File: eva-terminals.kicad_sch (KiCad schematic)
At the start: 24 parts, among them J1 RIBBON, J4 EXTRUDER, J5 HEATER, J6 SPI, J7 AUX, U1 LD39015M33R, U2 ADXL345

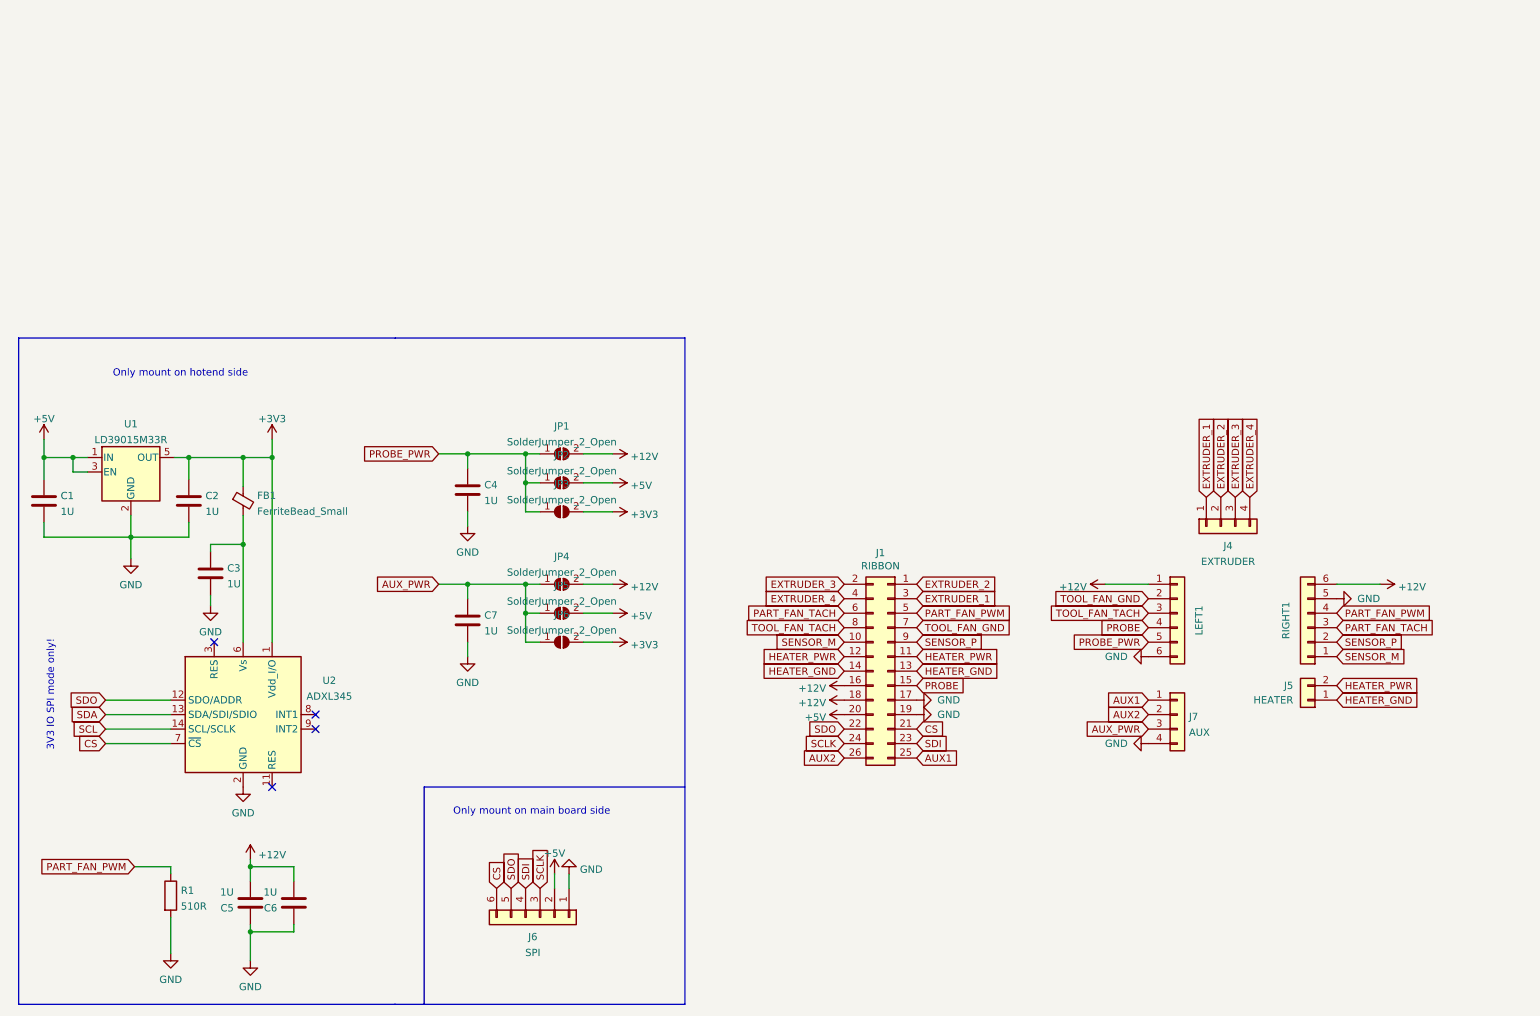
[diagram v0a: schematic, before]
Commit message: wip dual ribbon
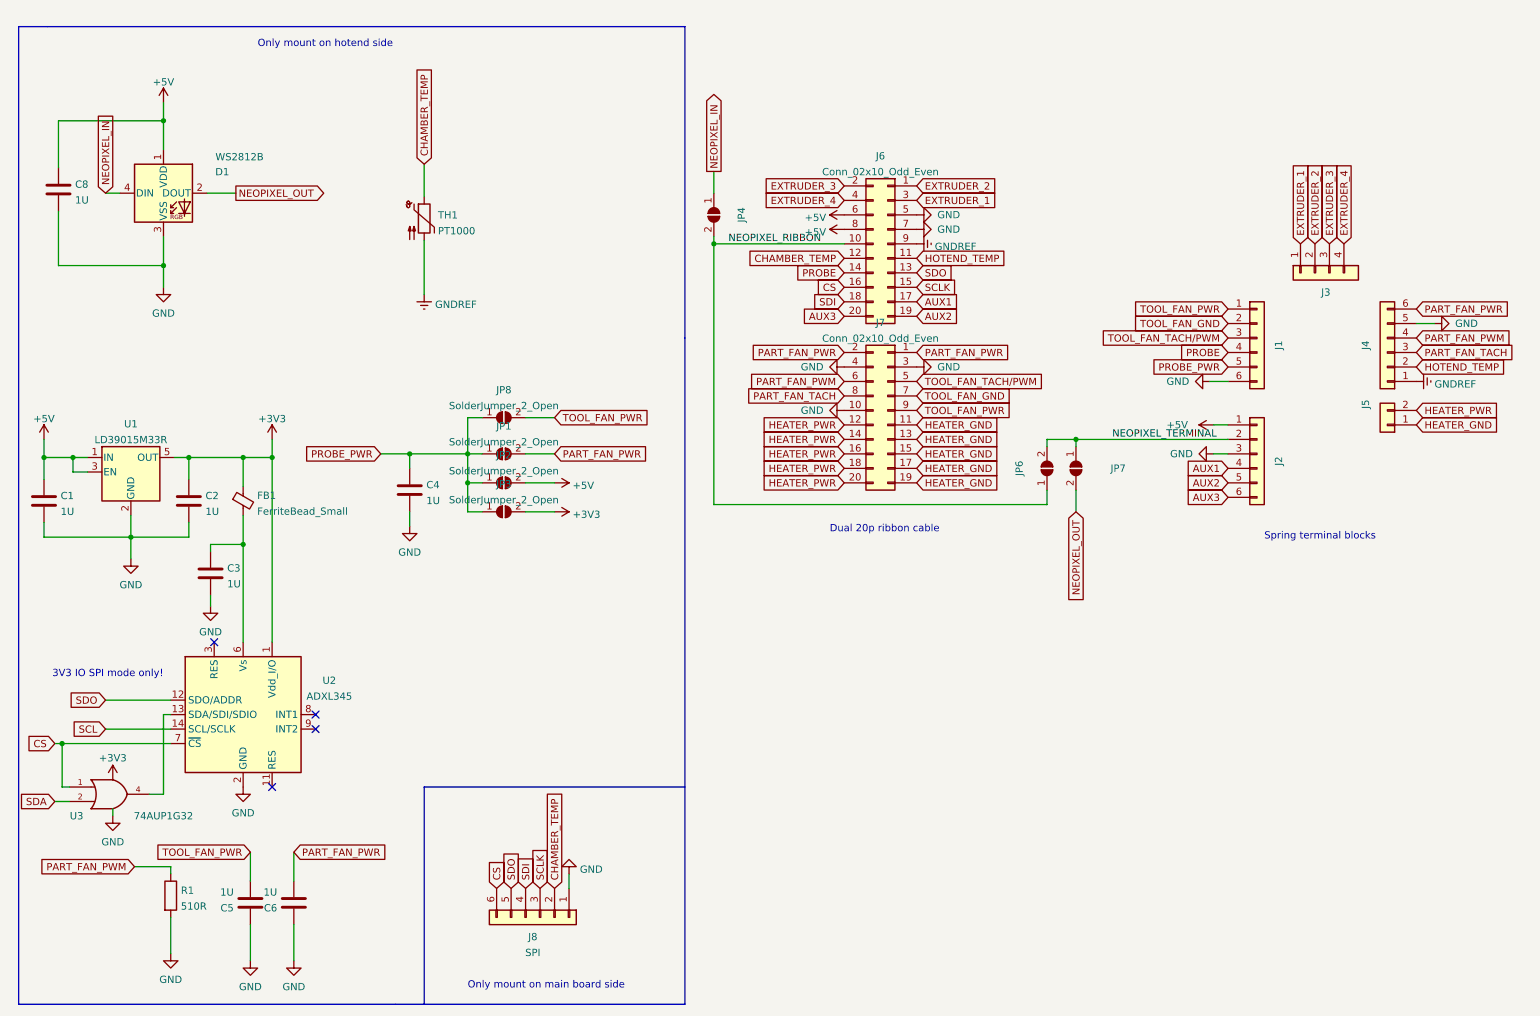
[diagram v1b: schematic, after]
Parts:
- removed C7: 1U, Capacitor_SMD:C_0805_2012Metric, symbol Device:C
- removed J1: RIBBON, Eagle_WR-MM (rev20b):690367292676, symbol Connector_Generic:Conn_02x13_Odd_Even
- removed J4: EXTRUDER, Eagle_WR-TBL Spring Clamp (rev21a):691402910004B, symbol eva-terminals:Conn_01x04_dual
- removed J7: AUX, Eagle_WR-TBL Spring Clamp (rev21a):691403900004B, symbol eva-terminals:Conn_01x04_dual
- removed JP5: SolderJumper_2_Open, Jumper:SolderJumper-2_P1.3mm_Open_RoundedPad1.0x1.5mm, symbol Jumper:SolderJumper_2_Open
- added C8: 1U, Capacitor_SMD:C_0805_2012Metric, symbol Device:C
- added D1: WS2812B, LED_SMD:LED_WS2812B_PLCC4_5.0x5.0mm_P3.2mm, symbol LED:WS2812B
- added J2: 691403900006B, Eagle_WR-TBL Spring Clamp (rev21a):691403900006B, symbol eva-terminals:Conn_01x06_dualpin
- added J3: Conn_01x04_dualpin, Eagle_WR-TBL Spring Clamp (rev21a):691402910004B, symbol eva-terminals:Conn_01x04_dualpin
- added J6, J7: Conn_02x10_Odd_Even, Eagle_WR-MM (rev20b):690367292076, symbol Connector_Generic:Conn_02x10_Odd_Even
- added JP7, JP8: SolderJumper_2_Open, Jumper:SolderJumper-2_P1.3mm_Open_RoundedPad1.0x1.5mm, symbol Jumper:SolderJumper_2_Open
- added TH1: PT1000, Resistor_SMD:R_1206_3216Metric, symbol Sensor_Temperature:PT1000
- added U3: 74AUP1G32, Package_TO_SOT_SMD:SOT-553, symbol 74xGxx:74AUP1G32
- renumbered LEFT1 to J1, RIGHT1 to J4, J6 to J8
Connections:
- net +3V3: now also U3.5 (VCC); no longer JP6.2 (B)
- net +5V: now also C8.1, D1.1 (VDD), J2.1 (Pin_1), J2.A1 (Pin_1A), J6.6 (Pin_6), J6.8 (Pin_8); no longer J8.2 (Pin_2), J8.A2 (Pin_A2)
- net AUX1: now also J2.4 (Pin_4), J2.A4 (Pin_A4), J6.17 (Pin_17)
- net AUX2: now also J2.5 (Pin_5), J2.A5 (Pin_A5), J6.19 (Pin_19)
- net CS: now also J6.16 (Pin_16), U3.1
- net EXTRUDER_1: now also J3.1 (Pin_1), J3.A1 (Pin_1A), J6.3 (Pin_3)
- net EXTRUDER_2: now also J3.2 (Pin_2), J3.A2 (Pin_A2), J6.1 (Pin_1)
- net EXTRUDER_3: now also J3.3 (Pin_3), J3.A3 (Pin_3), J6.2 (Pin_2)
- net EXTRUDER_4: now also J3.4 (Pin_4), J3.A4 (Pin_A4), J6.4 (Pin_4)
- net GND: now also C8.2, D1.3 (VSS), J2.3 (Pin_3), J2.A3 (Pin_3), J6.5 (Pin_5), J6.7 (Pin_7), J7.10 (Pin_10), J7.3 (Pin_3), J7.4 (Pin_4), U3.3 (GND)
- net HEATER_GND: now also J7.11 (Pin_11), J7.13 (Pin_13), J7.15 (Pin_15), J7.17 (Pin_17), J7.19 (Pin_19)
- net HEATER_PWR: now also J7.12 (Pin_12), J7.14 (Pin_14), J7.16 (Pin_16), J7.18 (Pin_18), J7.20 (Pin_20)
- net PART_FAN_PWM: now also J7.6 (Pin_6)
- net PART_FAN_TACH: now also J7.8 (Pin_8)
- net PROBE: now also J6.14 (Pin_14)
- net PROBE_PWR: now also JP8.1 (A)
- net SCLK: now also J6.15 (Pin_15)
- net SDA: now also U3.2; no longer U2.13 (SDA/SDI/SDIO)
- net SDI: now also J6.18 (Pin_18)
- net SDO: now also J6.13 (Pin_13)
- net TOOL_FAN_GND: now also J7.7 (Pin_7)
- net +12V renamed PART_FAN_PWR
- net PART_FAN_PWR: now also J7.1 (Pin_1), J7.2 (Pin_2); no longer C5.2, J1.1 (Pin_1), J1.A1 (Pin_1A), JP4.2 (B)
- net AUX_PWR renamed NEOPIXEL_IN
- net NEOPIXEL_IN: now also D1.4 (DIN); no longer JP6.1 (A)
- net SENSOR_M renamed GNDREF
- net GNDREF: now also J6.9 (Pin_9), TH1.2
- net SENSOR_P renamed HOTEND_TEMP
- net HOTEND_TEMP: now also J6.11 (Pin_11)
- net TOOL_FAN_TACH renamed TOOL_FAN_TACH/PWM
- net TOOL_FAN_TACH/PWM: now also J7.5 (Pin_5)
- new net: U2.13 (SDA/SDI/SDIO), U3.4
- new net AUX3: J2.6 (Pin_6), J2.A6 (Pin_A6), J6.20 (Pin_20)
- new net CHAMBER_TEMP: J6.12 (Pin_12), J8.2 (Pin_2), J8.A2 (Pin_A2), TH1.1
- new net NEOPIXEL_OUT: D1.2 (DOUT), JP7.2 (B)
- new net NEOPIXEL_RIBBON: J6.10 (Pin_10), JP4.2 (B), JP6.1 (A)
- new net NEOPIXEL_TERMINAL: J2.2 (Pin_2), J2.A2 (Pin_A2), JP6.2 (B), JP7.1 (A)
- new net TOOL_FAN_PWR: C5.2, J1.1 (Pin_1), J1.A1 (Pin_1A), J7.9 (Pin_9), JP8.2 (B)
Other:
- note added: "Dual 20p ribbon cable"
- note added: "Spring terminal blocks"
- moved on the sheet: C4, J1, J4, J5, JP1, JP2, JP3

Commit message: finalized board layout rev 1
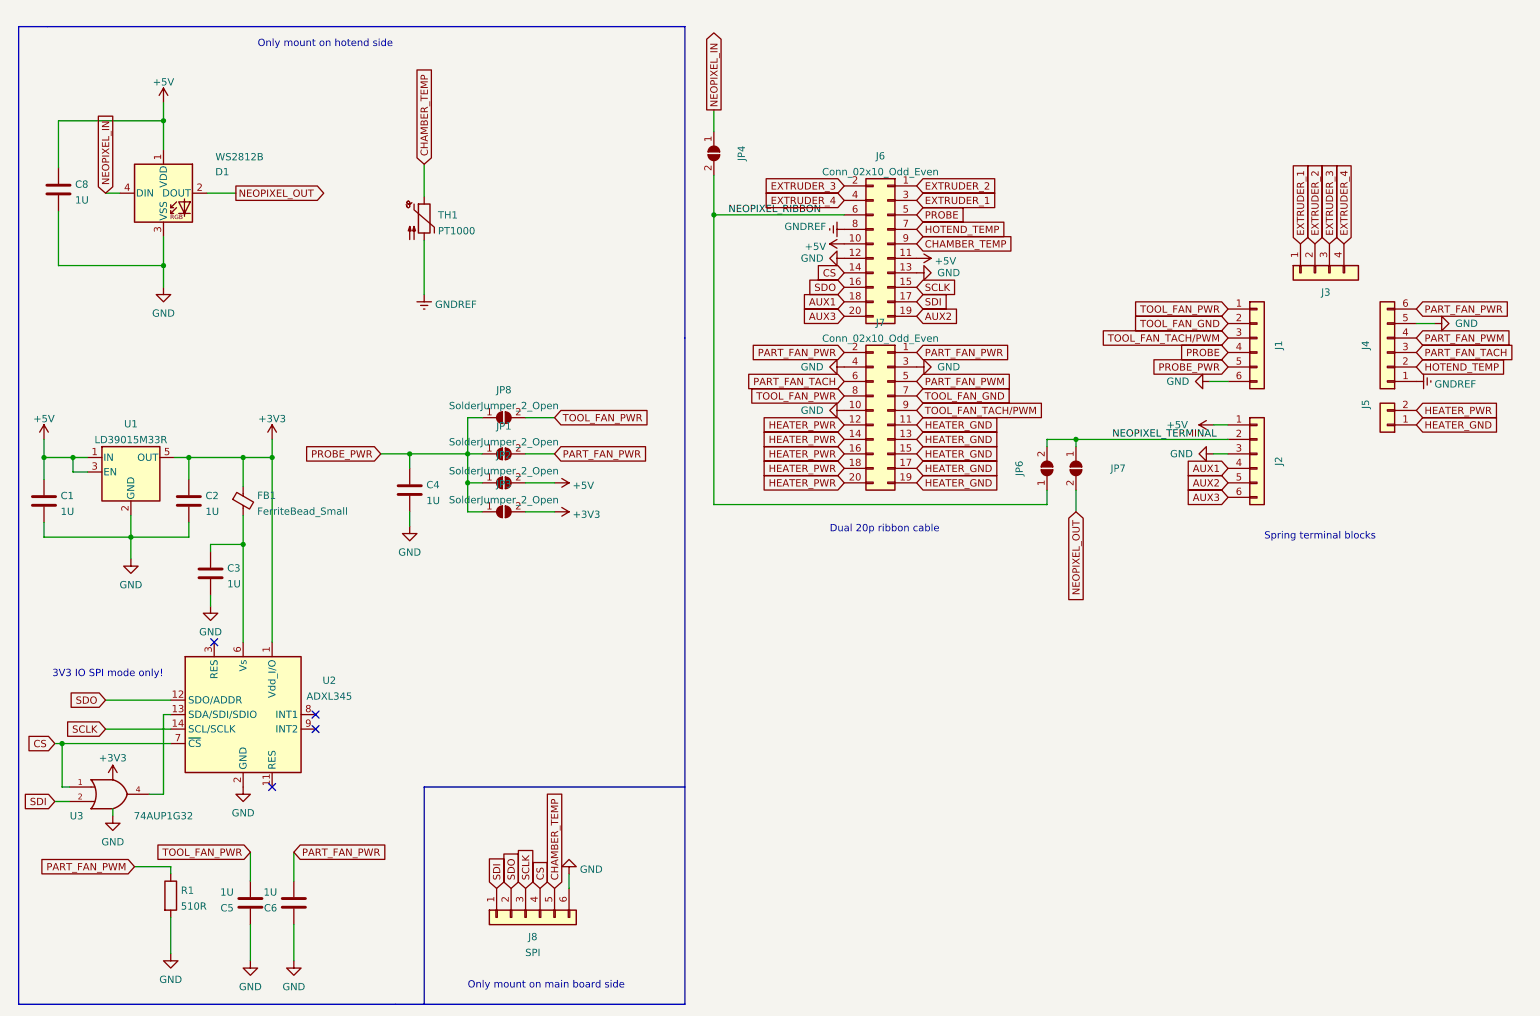
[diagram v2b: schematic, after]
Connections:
- net SCL is gone; now on net SCLK: U2.14 (SCL/SCLK)
- net SDA is gone; now on net SDI: U3.2
- net +5V: now also J6.10 (Pin_10), J6.11 (Pin_11); no longer J6.6 (Pin_6), J6.8 (Pin_8)
- net AUX1: now also J6.18 (Pin_18); no longer J6.17 (Pin_17)
- net CHAMBER_TEMP: now also J6.9 (Pin_9), J8.5 (Pin_5), J8.A5 (Pin_A5); no longer J6.12 (Pin_12), J8.2 (Pin_2), J8.A2 (Pin_A2)
- net CS: now also J6.14 (Pin_14), J8.4 (Pin_4), J8.A4 (Pin_A4); no longer J6.16 (Pin_16), J8.6 (Pin_6), J8.A6 (Pin_A6)
- net GND: now also J6.12 (Pin_12), J6.13 (Pin_13), J8.6 (Pin_6), J8.A6 (Pin_A6); no longer J6.5 (Pin_5), J6.7 (Pin_7), J8.1 (Pin_1), J8.A1 (Pin_1A)
- net GNDREF: now also J6.8 (Pin_8); no longer J6.9 (Pin_9)
- net HOTEND_TEMP: now also J6.7 (Pin_7); no longer J6.11 (Pin_11)
- net NEOPIXEL_RIBBON: now also J6.6 (Pin_6); no longer J6.10 (Pin_10)
- net PART_FAN_PWM: now also J7.5 (Pin_5); no longer J7.6 (Pin_6)
- net PART_FAN_TACH: now also J7.6 (Pin_6); no longer J7.8 (Pin_8)
- net PROBE: now also J6.5 (Pin_5); no longer J6.14 (Pin_14)
- net SDI: now also J6.17 (Pin_17), J8.1 (Pin_1), J8.A1 (Pin_1A); no longer J6.18 (Pin_18), J8.4 (Pin_4), J8.A4 (Pin_A4)
- net SDO: now also J6.16 (Pin_16), J8.2 (Pin_2), J8.A2 (Pin_A2); no longer J6.13 (Pin_13), J8.5 (Pin_5), J8.A5 (Pin_A5)
- net TOOL_FAN_PWR: now also J7.8 (Pin_8); no longer J7.9 (Pin_9)
- net TOOL_FAN_TACH/PWM: now also J7.9 (Pin_9); no longer J7.5 (Pin_5)
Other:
- moved on the sheet: J8, JP4
